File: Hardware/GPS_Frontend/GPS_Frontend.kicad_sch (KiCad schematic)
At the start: 34 parts, among them J1 Pmod, J2 Passive ANT, J3 Active ANT, SW1 SW_DIP_x02, SW2 SW_DIP_x01, U1 MAX2769ETI_, U2 TPS7A2030PDBVR, U3 TPS7A2030PDBVR, Y1 19.2 Mhz

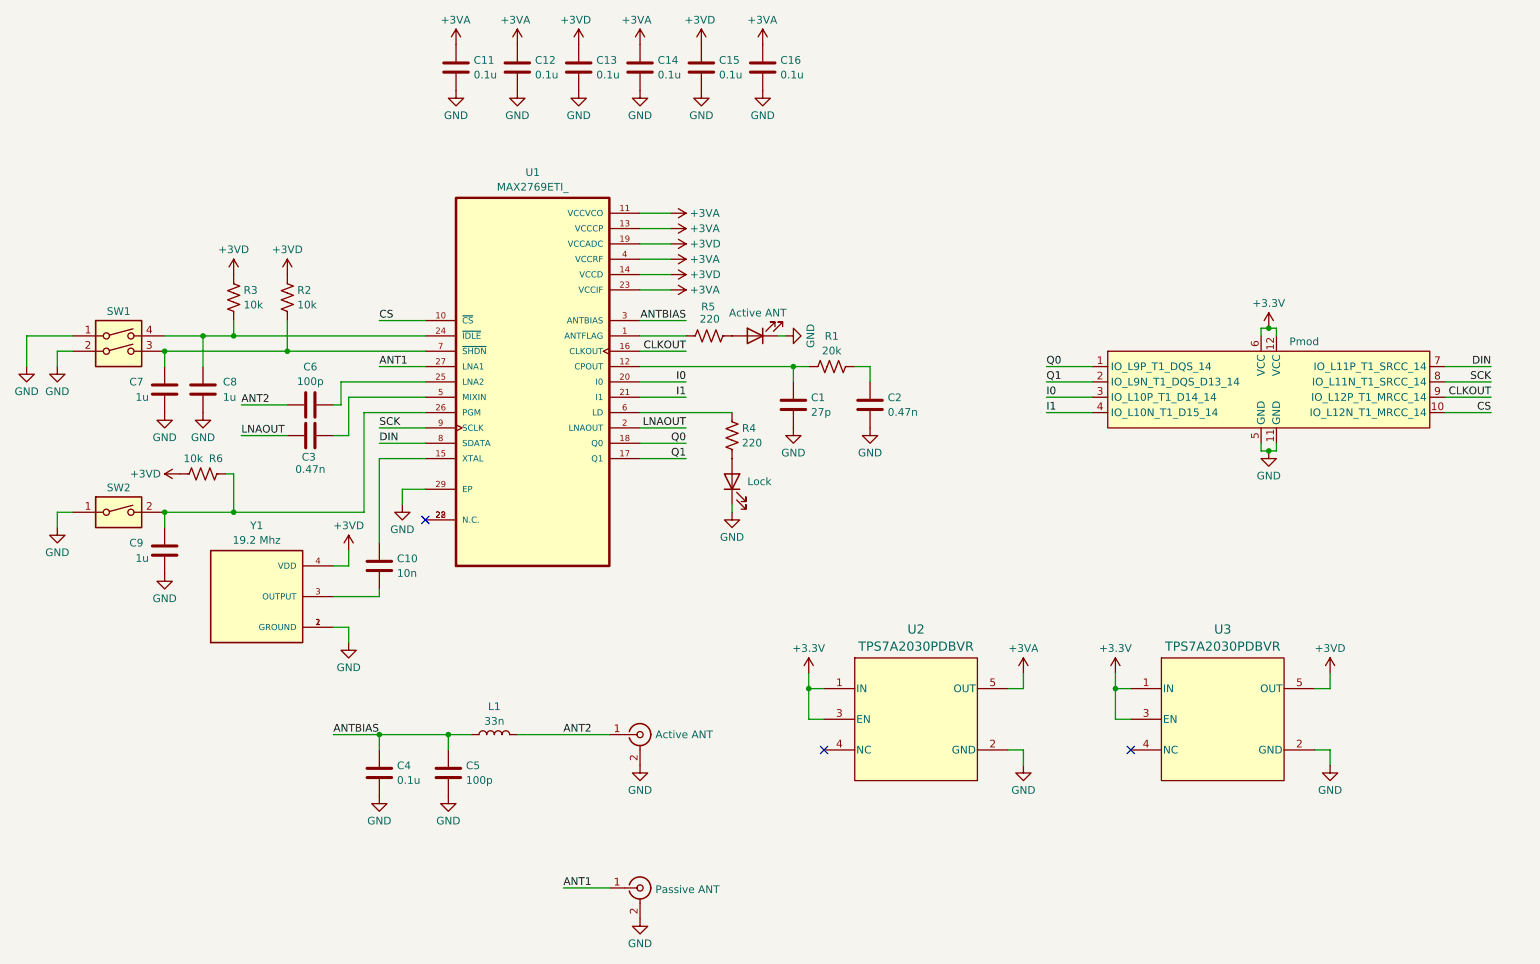
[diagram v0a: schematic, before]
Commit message: Version submitted for manufacturing
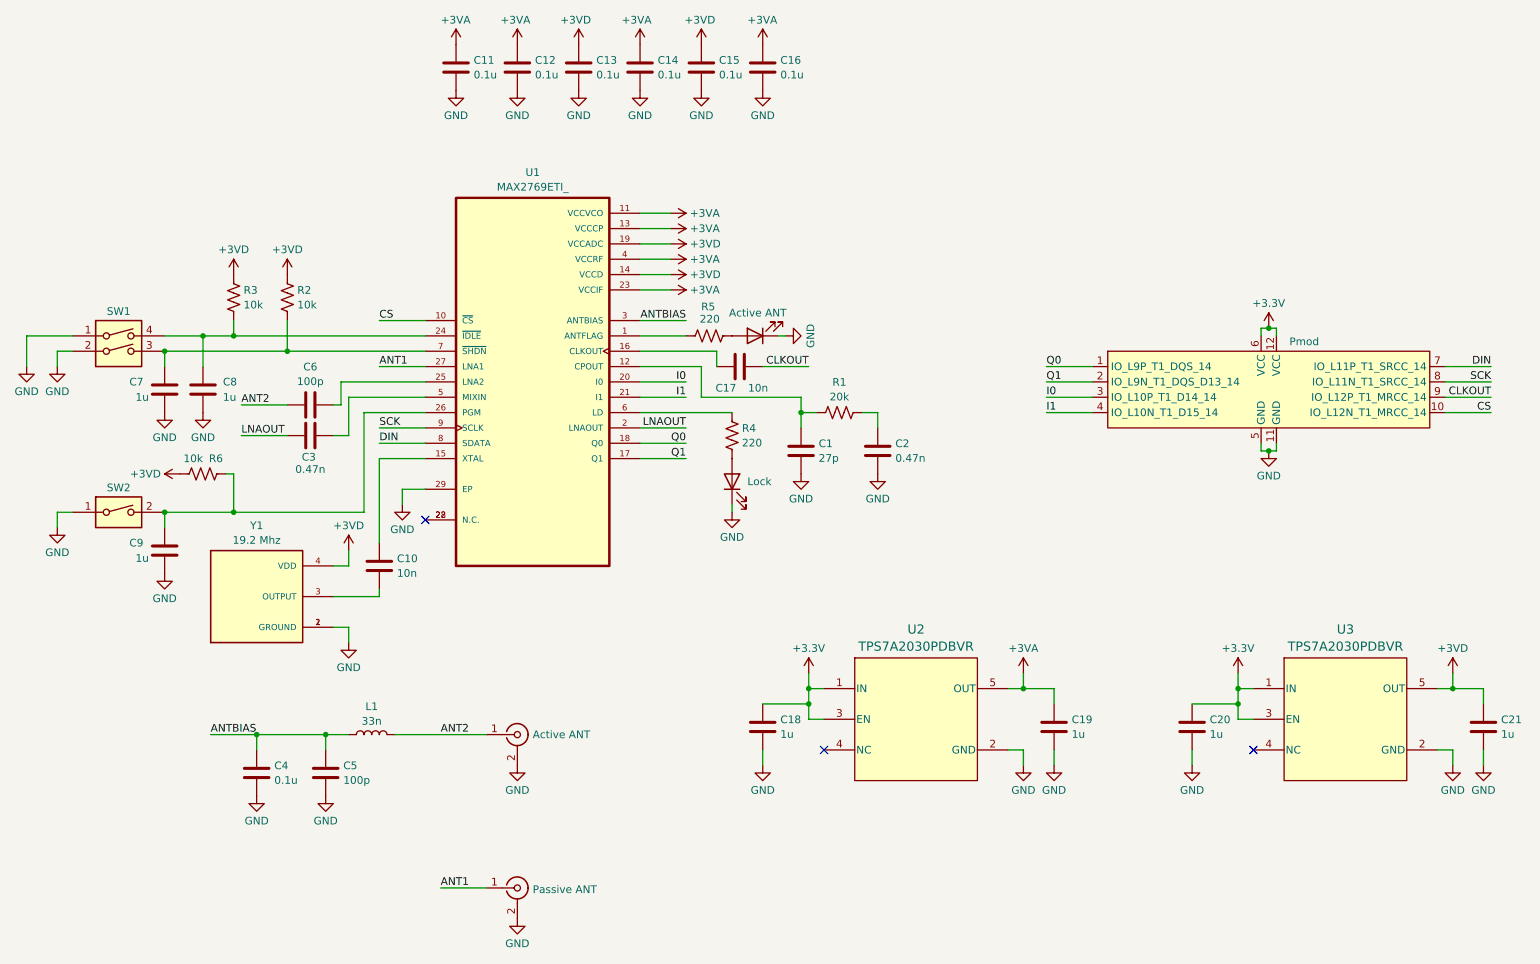
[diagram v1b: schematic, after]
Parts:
- added C17: 10n, Capacitor_SMD:C_0603_1608Metric, symbol Device:C
- added C18, C19, C20, C21: 1u, Capacitor_SMD:C_0603_1608Metric, symbol Device:C
- C1: Manufacturer_Part_Number (none) -> GCM1555C1H270JA16J
- C10: Manufacturer_Part_Number (none) -> GCM188R72A103KA37D
- C11, C12, C13, C14, C15, C16, C4: Manufacturer_Part_Number (none) -> GRM155R61A104KA01J
- C2, C3: Manufacturer_Part_Number (none) -> GCM1555C1H471JA16J
- C5, C6: Manufacturer_Part_Number (none) -> GRM1555C2A101GA01D
- C7, C8, C9: Manufacturer_Part_Number (none) -> GRM188R61A105KA61J
- J1: Manufacturer_Part_Number (none) -> HTSW-106-08-G-D-RA
- J2, J3: Manufacturer_Part_Number (none) -> 60312242114510
- L1: Manufacturer_Part_Number (none) -> LQW15AN33NJ80D
- LED1: Manufacturer_Part_Number (none) -> 150080VS75000
- LED2: Manufacturer_Part_Number (none) -> 150080RS75000
- R1: Manufacturer_Part_Number (none) -> RT0603FRE1020KL
- R2, R3, R6: Manufacturer_Part_Number (none) -> RE0603FRE1310KL
- R4, R5: Manufacturer_Part_Number (none) -> RC0603JR-07220RP
- SW1: Manufacturer_Part_Number (none) -> A6S-2104-H
- SW2: Manufacturer_Part_Number (none) -> A6S-1104-H
- U1: Manufacturer_Part_Number (none) -> MAX2769ETI
- U2, U3: Manufacturer_Part_Number (none) -> TPS7A2030PDBVR
- Y1: Manufacturer_Part_Number (none) -> ECS-TXO-20CSMV4-192-AN-TR
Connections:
- net +3.3V: now also C18.1, C20.1
- net +3VA: now also C19.1
- net +3VD: now also C21.1
- net CLKOUT: now also C17.2; no longer U1.16 (CLKOUT)
- net GND: now also C18.2, C19.2, C20.2, C21.2
- new net: C17.1, U1.16 (CLKOUT)
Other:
- moved on the sheet: C1, C2, C4, C5, L1, R1, U3
